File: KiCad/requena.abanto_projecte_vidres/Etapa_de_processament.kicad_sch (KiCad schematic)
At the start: 43 parts, among them J1 Conn_01x05, J3 DE9_Pins, J4 DE9_Pins, J6 Conn_01x04, SW1 SW_Push_SPDT, SW2 SW_Push, SW3 SW_Omron_B3FS, SW4 SW_Omron_B3FS, SW5 SW_Omron_B3FS, SW6 SW_Omron_B3FS, U6 PIC24HJ128GP502, U7 PN5120A0HN1, U9 TJA1051TK-3, Y1 27.12 MHz, Y2 8 MHz

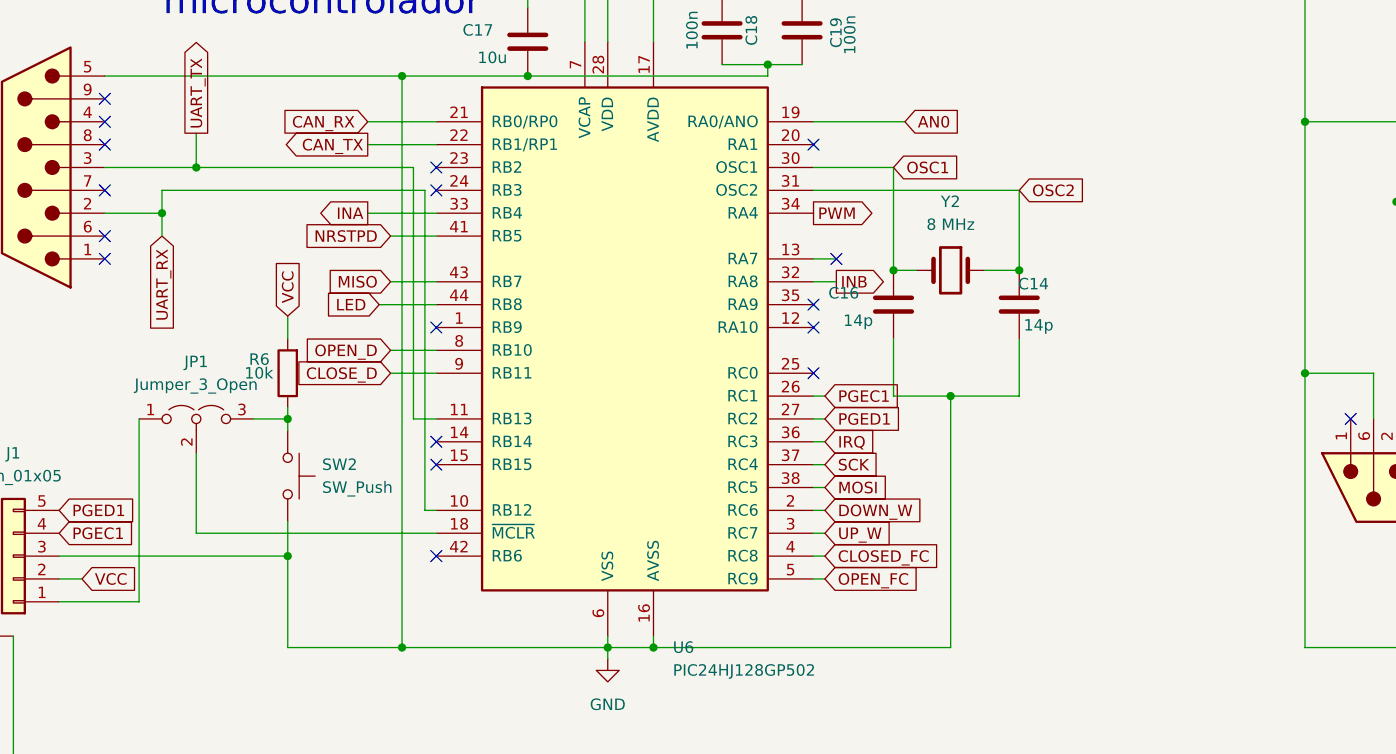
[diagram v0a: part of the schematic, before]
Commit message: buenas noches alfred
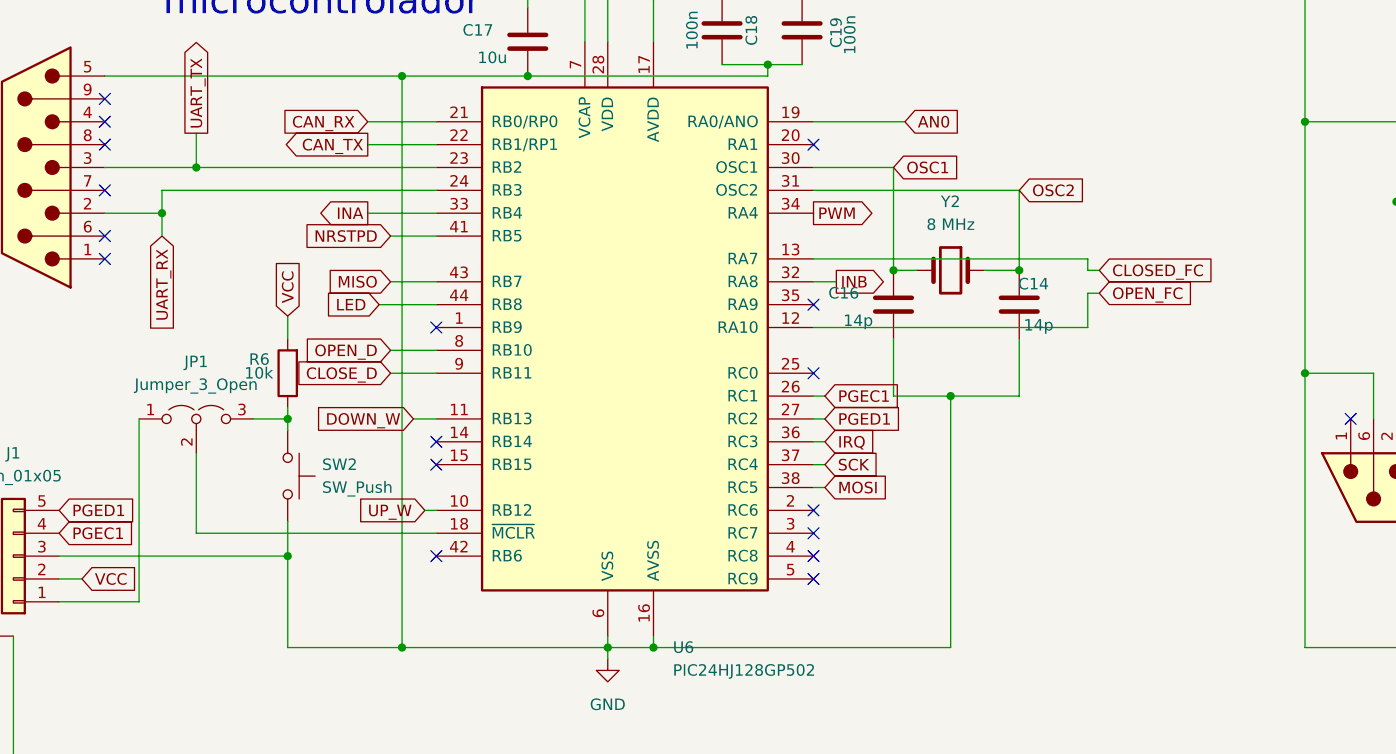
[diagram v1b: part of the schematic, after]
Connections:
- net CLOSED_FC: now also U6.13 (RA7); no longer U6.4 (RC8)
- net DOWN_W: now also U6.11 (RB13); no longer U6.2 (RC6)
- net OPEN_FC: now also U6.12 (RA10); no longer U6.5 (RC9)
- net UART_RX: now also U6.24 (RB3); no longer U6.10 (RB12)
- net UART_TX: now also U6.23 (RB2); no longer U6.11 (RB13)
- net UP_W: now also U6.10 (RB12); no longer U6.3 (RC7)

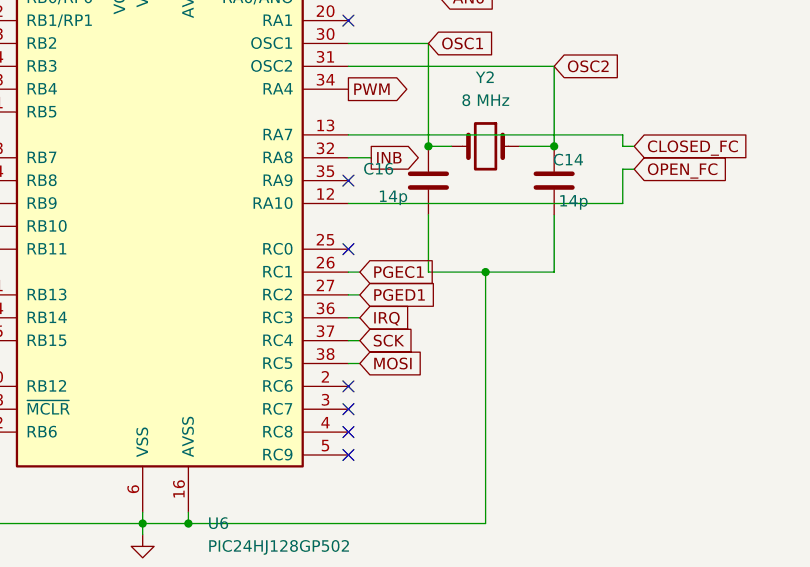
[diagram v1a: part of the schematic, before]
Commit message: Placement més o menys colocat, i avenç de algunes connexions
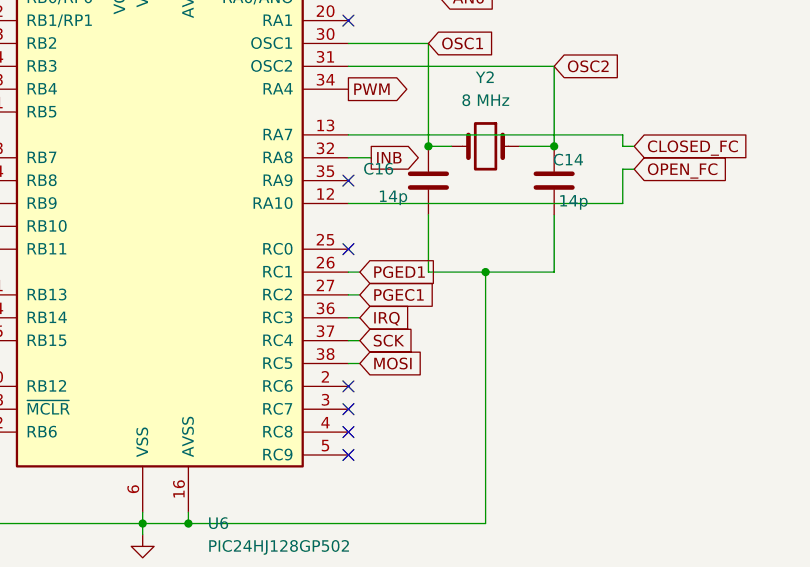
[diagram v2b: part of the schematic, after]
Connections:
- net PGEC1: now also U6.27 (RC2); no longer U6.26 (RC1)
- net PGED1: now also U6.26 (RC1); no longer U6.27 (RC2)

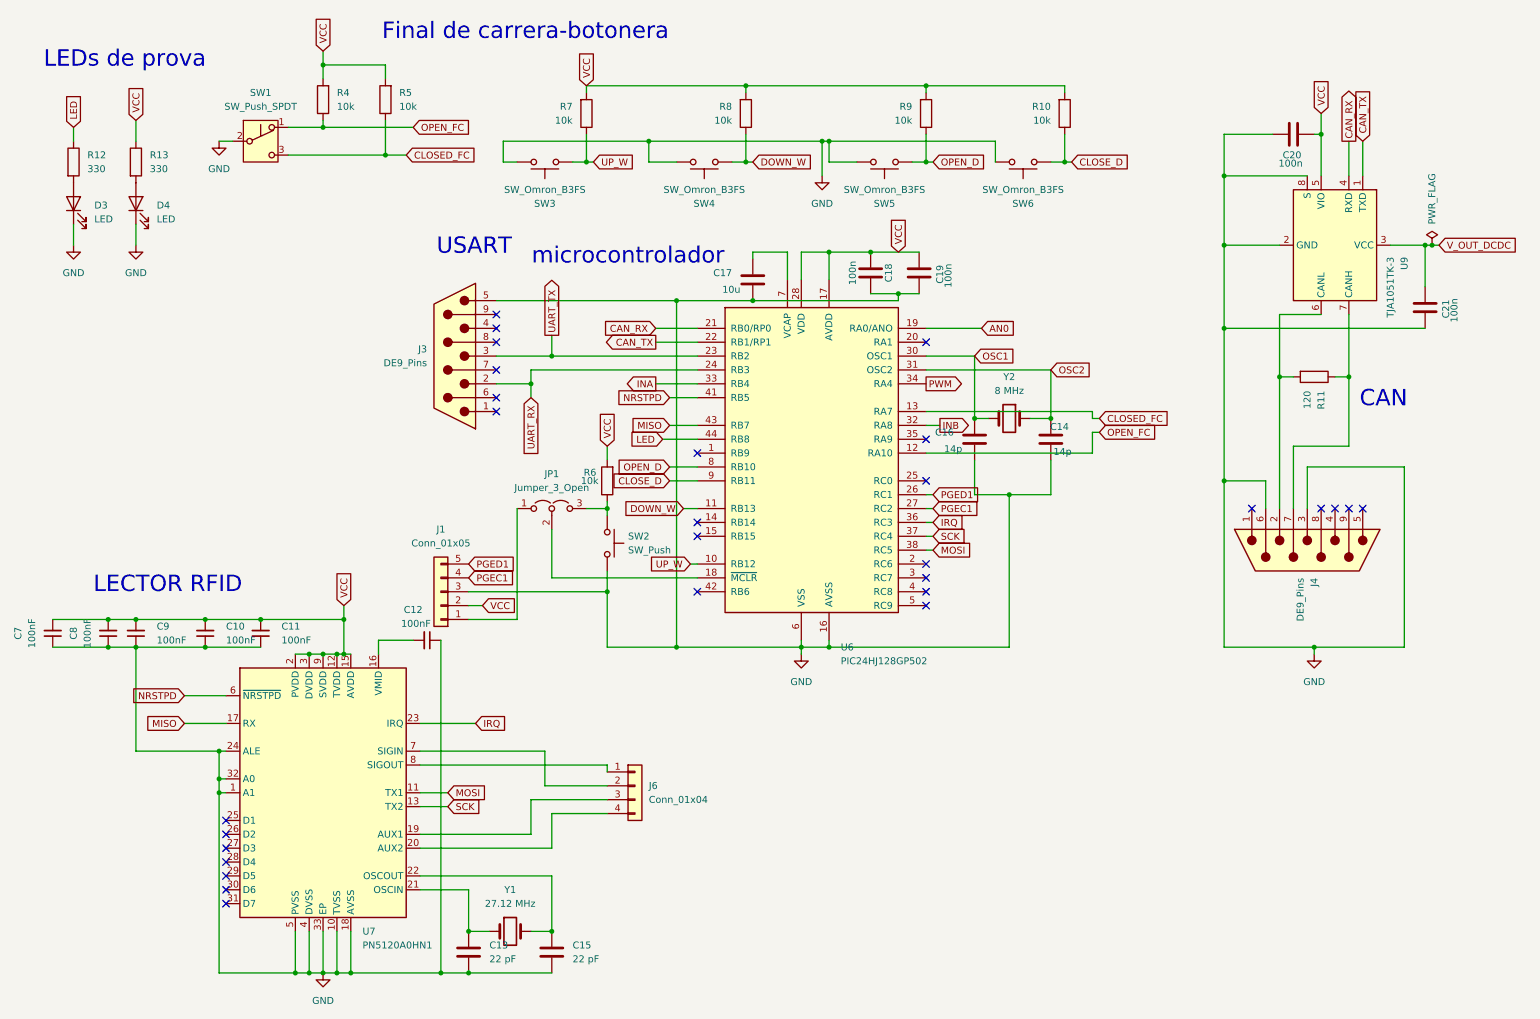
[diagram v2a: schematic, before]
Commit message: el RFID me jodio la vida
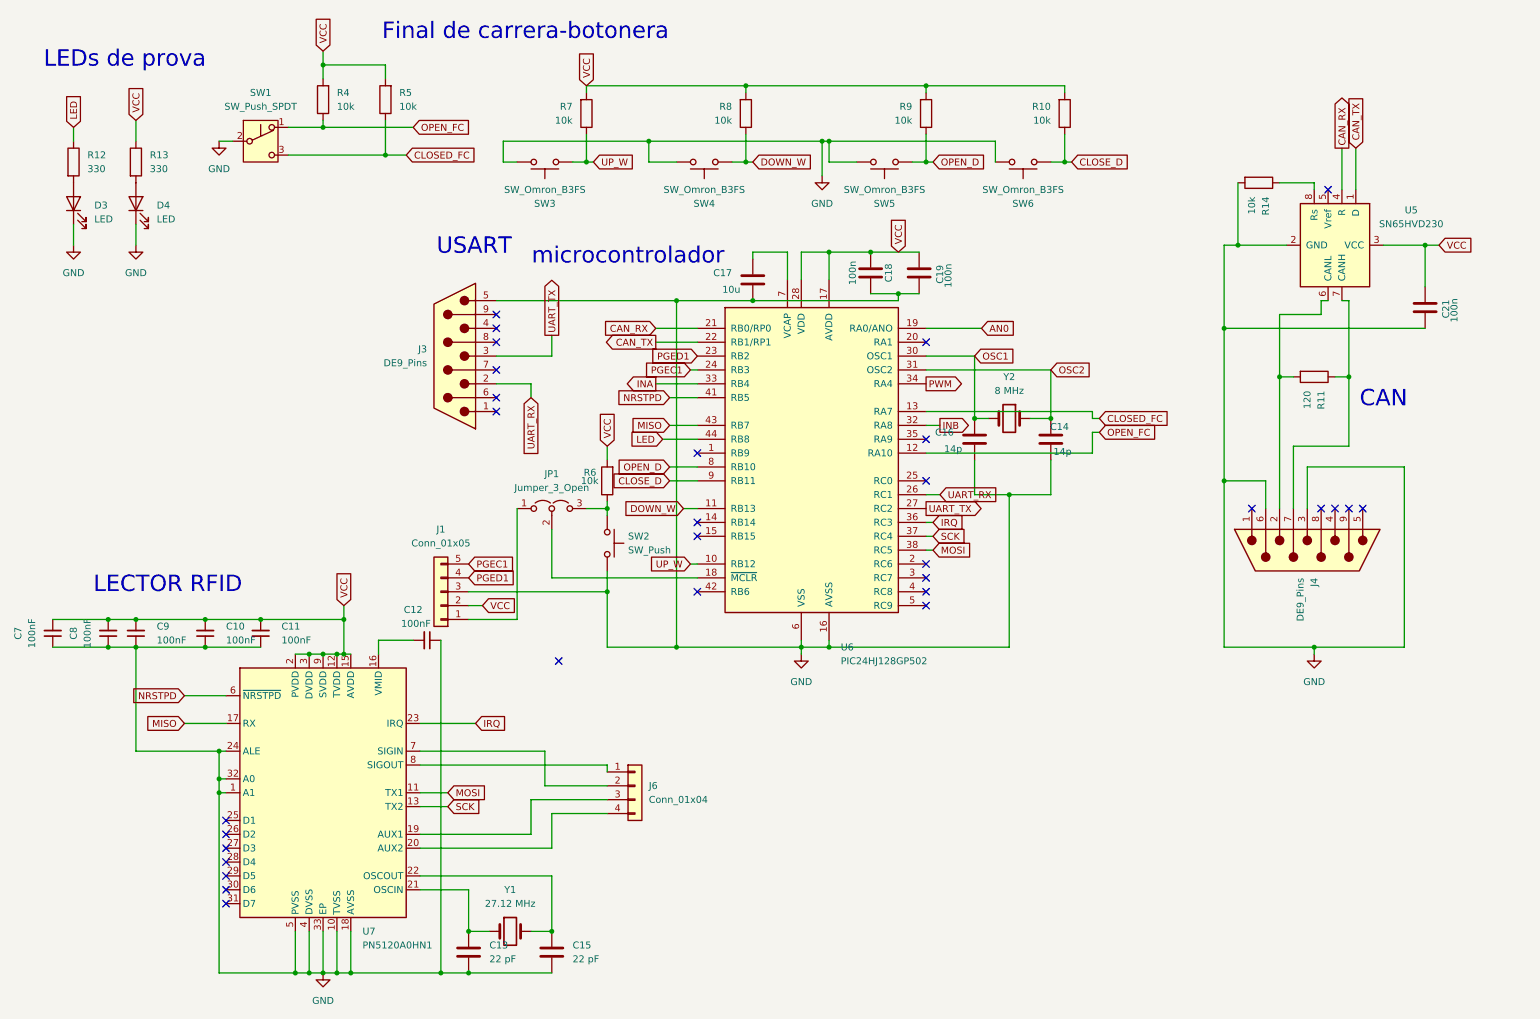
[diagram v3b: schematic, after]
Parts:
- removed C20: 100n, Capacitor_SMD:C_1206_3216Metric, symbol Device:C
- removed U9: TJA1051TK-3, Package_SON:HVSON-8-1EP_3x3mm_P0.65mm_EP1.6x2.4mm, symbol Interface_CAN_LIN:TJA1051TK-3
- added R14: 10k, Resistor_SMD:R_1206_3216Metric, symbol Device:R
- added U5: SN65HVD230, Package_SO:SOIC-8_3.9x4.9mm_P1.27mm, symbol Interface_CAN_LIN:SN65HVD230
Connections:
- net V_OUT_DCDC is gone; now on net VCC: C21.1
- net CAN_RX: now also U5.4 (R)
- net CAN_TX: now also U5.1 (D)
- net GND: now also R14.2, U5.2 (GND)
- net PGEC1: now also J1.5 (Pin_5), U6.24 (RB3); no longer J1.4 (Pin_4), U6.27 (RC2)
- net PGED1: now also J1.4 (Pin_4), U6.23 (RB2); no longer J1.5 (Pin_5), U6.26 (RC1)
- net UART_RX: now also U6.26 (RC1); no longer U6.24 (RB3)
- net UART_TX: now also U6.27 (RC2); no longer U6.23 (RB2)
- net VCC: now also U5.3 (VCC)
- net at J4.2, R11.2: now also U5.6 (CANL)
- net at J4.7, R11.1: now also U5.7 (CANH)
- new net: R14.1, U5.8 (Rs)
- no-connect marks 29 -> 31
